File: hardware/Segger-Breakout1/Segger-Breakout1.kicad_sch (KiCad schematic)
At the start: 5 parts, among them J1 GND, J2 Breakout, J3 SWD Mini IDC, J4 JLink IDC, J6 RP2040

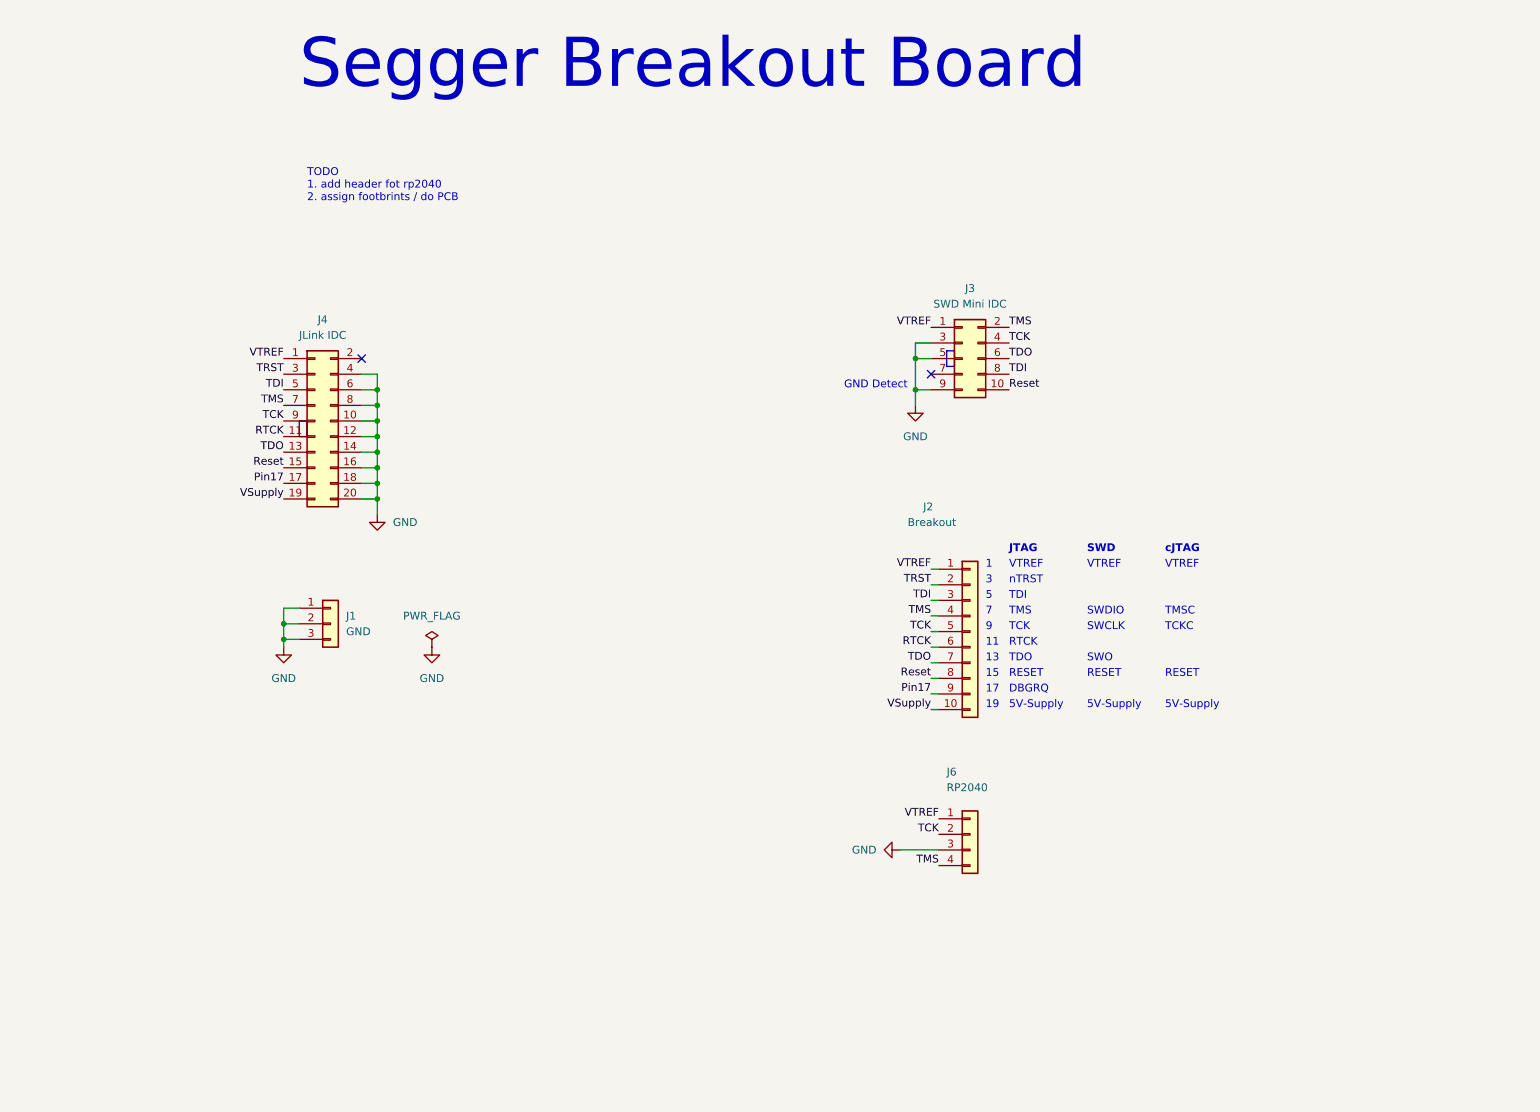
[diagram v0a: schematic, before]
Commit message: updates
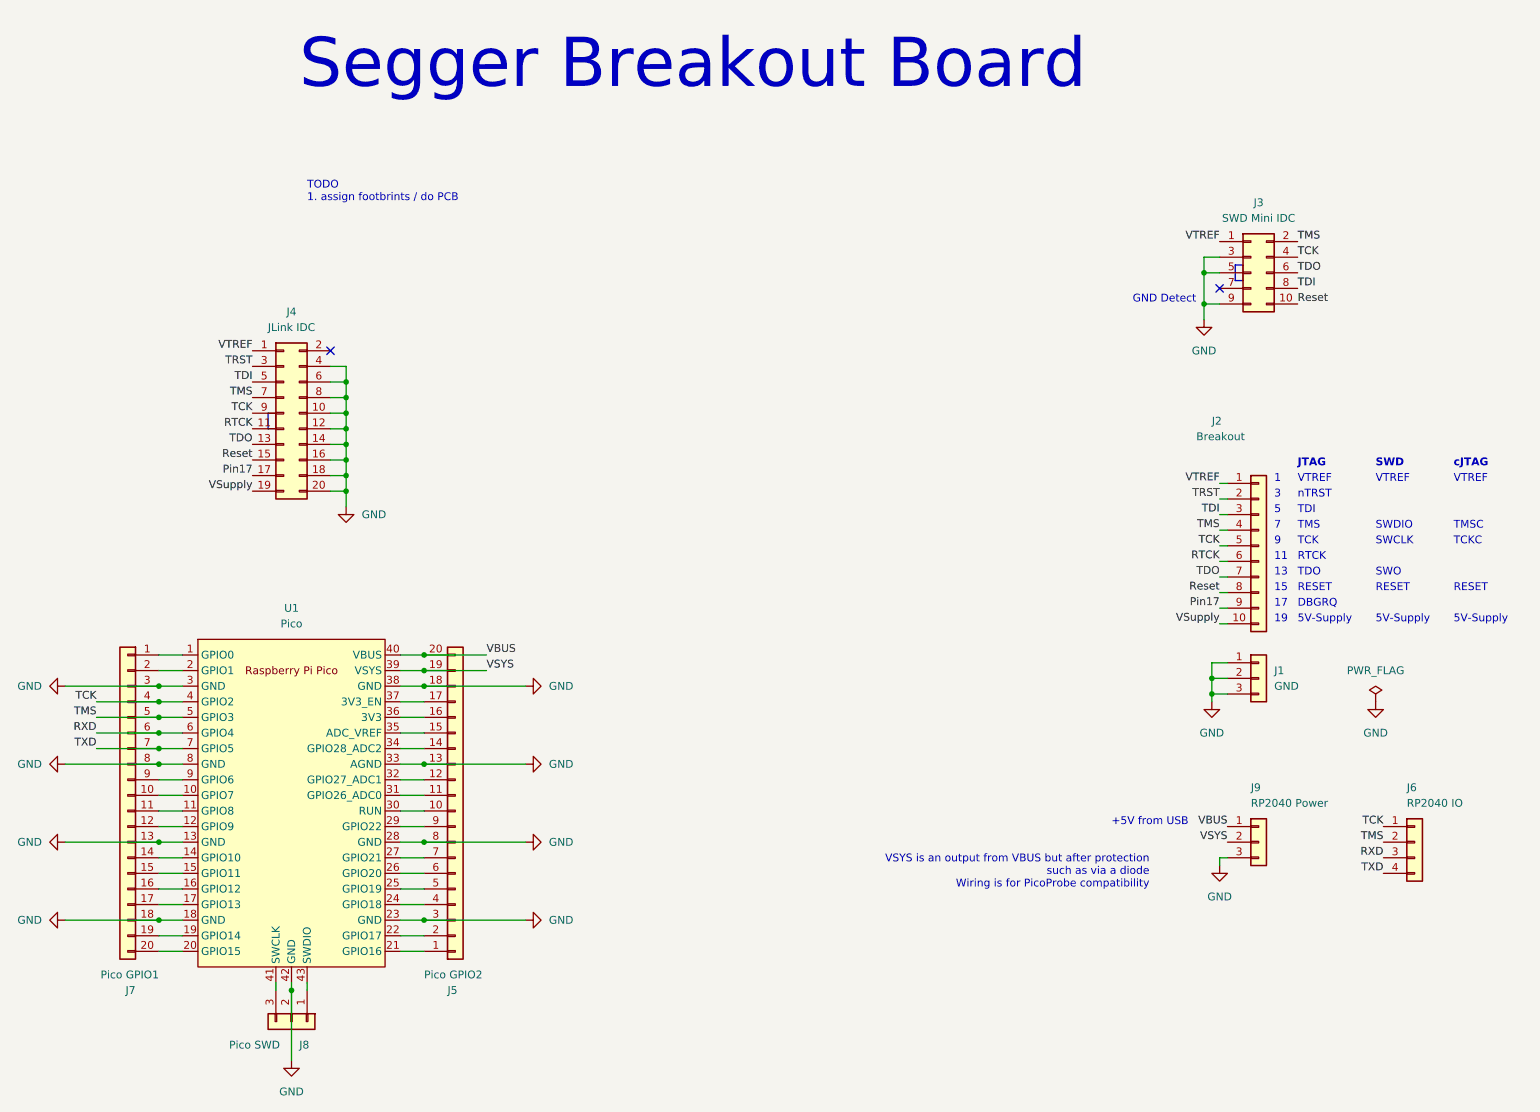
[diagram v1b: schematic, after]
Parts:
- added J5: Pico GPIO2, Connector_PinHeader_2.54mm:PinHeader_1x20_P2.54mm_Vertical, symbol Connector_Generic:Conn_01x20
- added J7: Pico GPIO1, Connector_PinHeader_2.54mm:PinHeader_1x20_P2.54mm_Vertical, symbol Connector_Generic:Conn_01x20
- added J8: Pico SWD, Connector_PinHeader_2.54mm:PinHeader_1x03_P2.54mm_Vertical, symbol Connector_Generic:Conn_01x03
- added J9: RP2040 Power, Connector_PinHeader_2.54mm:PinHeader_1x03_P2.54mm_Vertical, symbol Connector_Generic:Conn_01x03
- added U1: Pico, MCU_RaspberryPi_and_Boards:RPi_Pico_SMD_TH, symbol MCU_RaspberryPi_and_Boards:Pico
- J6: value RP2040 -> RP2040 IO
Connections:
- net GND: now also J5.13 (Pin_13), J5.18 (Pin_18), J5.3 (Pin_3), J5.8 (Pin_8), J7.13 (Pin_13), J7.18 (Pin_18), J7.3 (Pin_3), J7.8 (Pin_8), J8.2 (Pin_2), J9.3 (Pin_3), U1.13 (GND), U1.18 (GND), U1.23 (GND), U1.28 (GND), U1.3 (GND), U1.33 (AGND), U1.38 (GND), U1.42 (GND), U1.8 (GND); no longer J6.3 (Pin_3)
- net TCK: now also J6.1 (Pin_1), J7.4 (Pin_4), U1.4 (GPIO2); no longer J6.2 (Pin_2)
- net TMS: now also J6.2 (Pin_2), J7.5 (Pin_5), U1.5 (GPIO3); no longer J6.4 (Pin_4)
- net VTREF: no longer J6.1 (Pin_1)
- new net: J7.1 (Pin_1), U1.1 (GPIO0)
- new net: J7.10 (Pin_10), U1.10 (GPIO7)
- new net: J7.11 (Pin_11), U1.11 (GPIO8)
- new net: J7.12 (Pin_12), U1.12 (GPIO9)
- new net: J7.14 (Pin_14), U1.14 (GPIO10)
- new net: J7.15 (Pin_15), U1.15 (GPIO11)
- new net: J7.16 (Pin_16), U1.16 (GPIO12)
- new net: J7.17 (Pin_17), U1.17 (GPIO13)
- new net: J7.19 (Pin_19), U1.19 (GPIO14)
- new net: J7.2 (Pin_2), U1.2 (GPIO1)
- new net: J7.20 (Pin_20), U1.20 (GPIO15)
- new net: J7.9 (Pin_9), U1.9 (GPIO6)
- new net: J5.1 (Pin_1), U1.21 (GPIO16)
- new net: J5.2 (Pin_2), U1.22 (GPIO17)
- new net: J5.4 (Pin_4), U1.24 (GPIO18)
- new net: J5.5 (Pin_5), U1.25 (GPIO19)
- new net: J5.6 (Pin_6), U1.26 (GPIO20)
- new net: J5.7 (Pin_7), U1.27 (GPIO21)
- new net: J5.9 (Pin_9), U1.29 (GPIO22)
- new net: J5.10 (Pin_10), U1.30 (RUN)
- new net: J5.11 (Pin_11), U1.31 (GPIO26_ADC0)
- new net: J5.12 (Pin_12), U1.32 (GPIO27_ADC1)
- new net: J5.14 (Pin_14), U1.34 (GPIO28_ADC2)
- new net: J5.15 (Pin_15), U1.35 (ADC_VREF)
- new net: J5.16 (Pin_16), U1.36 (3V3)
- new net: J5.17 (Pin_17), U1.37 (3V3_EN)
- new net: J8.3 (Pin_3), U1.41 (SWCLK)
- new net: J8.1 (Pin_1), U1.43 (SWDIO)
- new net RXD: J6.3 (Pin_3), J7.6 (Pin_6), U1.6 (GPIO4)
- new net TXD: J6.4 (Pin_4), J7.7 (Pin_7), U1.7 (GPIO5)
- new net VBUS: J5.20 (Pin_20), J9.1 (Pin_1), U1.40 (VBUS)
- new net VSYS: J5.19 (Pin_19), J9.2 (Pin_2), U1.39 (VSYS)
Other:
- note added: "+5V from USB"
- note added: "TODO 1. assign footbrints / do PCB"
- note added: "VSYS is an output from VBUS but after protection such as via a diode Wiring is for PicoProbe compatibility"
- note removed: "TODO 1. add header fot rp2040 2. assign footbrints / do PCB"
- moved on the sheet: J1, J2, J3, J4, J6
